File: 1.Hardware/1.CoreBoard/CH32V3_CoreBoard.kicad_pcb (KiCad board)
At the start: 4 copper layers, 38.2 x 25.2 mm, 55 parts, among them J2 SH1.0_4P, J4 BTB_02X18, J5 BTB_02X18, SW1 3x4, SW2 3x4, SW3 3x4, SW4 3x4, U2 RT9013-33GB, U3 BMI270, U5 IPS096, Y1 32.768KHz, Y2 8MHz

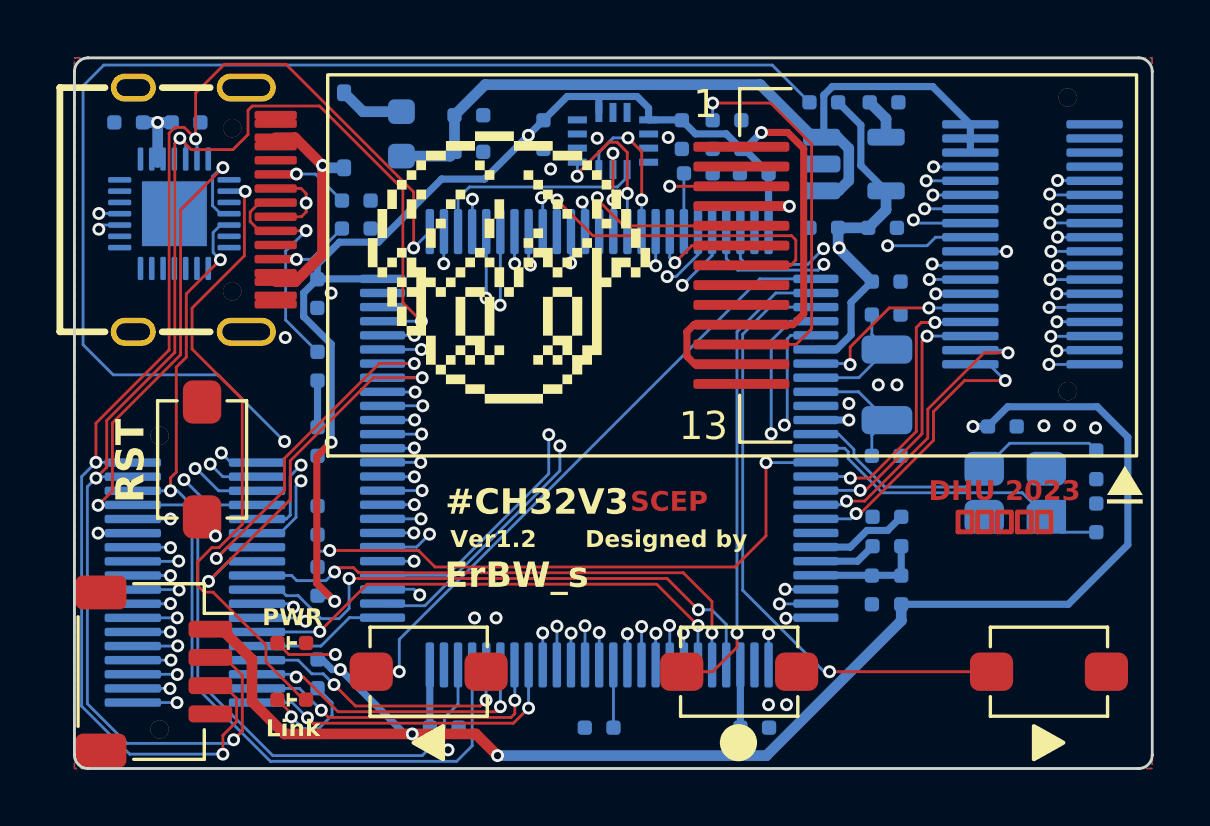
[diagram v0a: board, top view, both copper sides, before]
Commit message: Fix CoreBoard for production
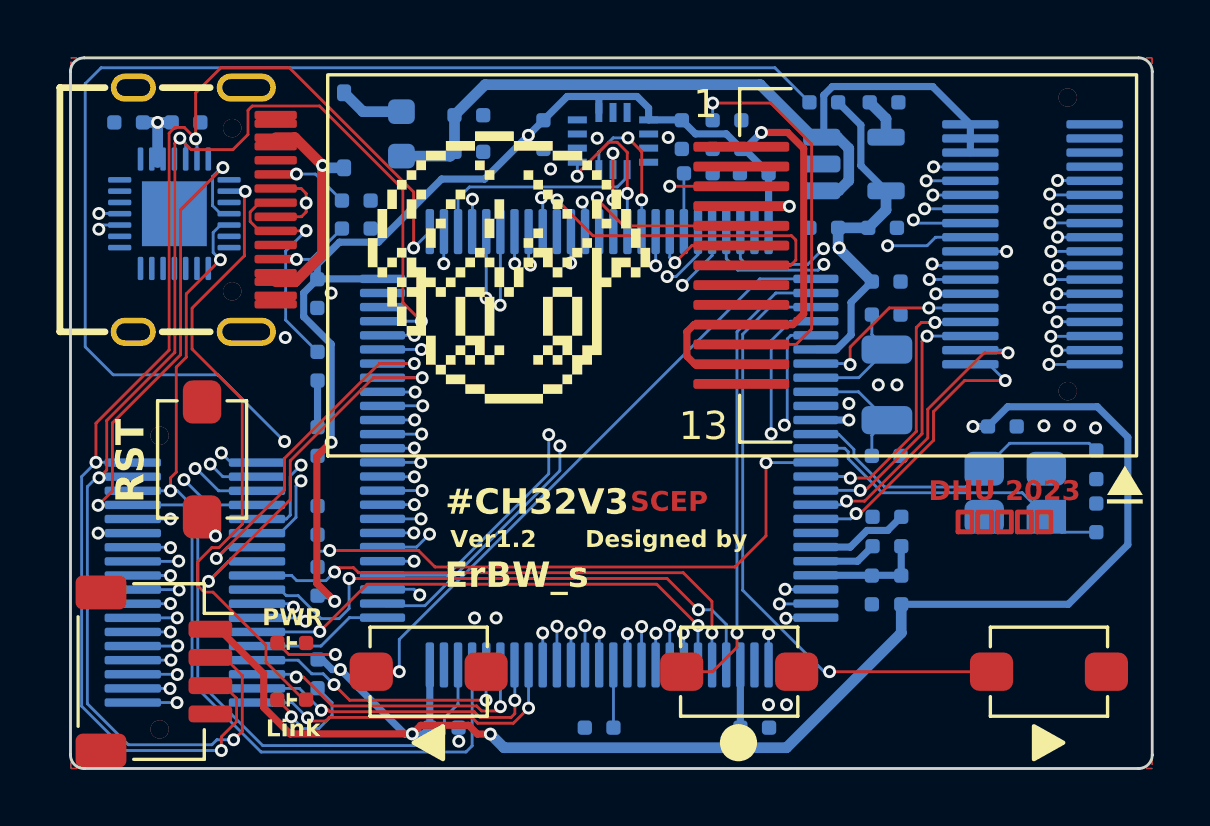
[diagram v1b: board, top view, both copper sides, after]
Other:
- board size 38.2 x 25.2 mm -> 38.3 x 25.2 mm
